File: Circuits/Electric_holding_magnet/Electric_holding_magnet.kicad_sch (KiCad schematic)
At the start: 9 parts, among them J1 Conn_01x03, Q1 BC547, Q2 BC547, SW1 SW_DIP_x01

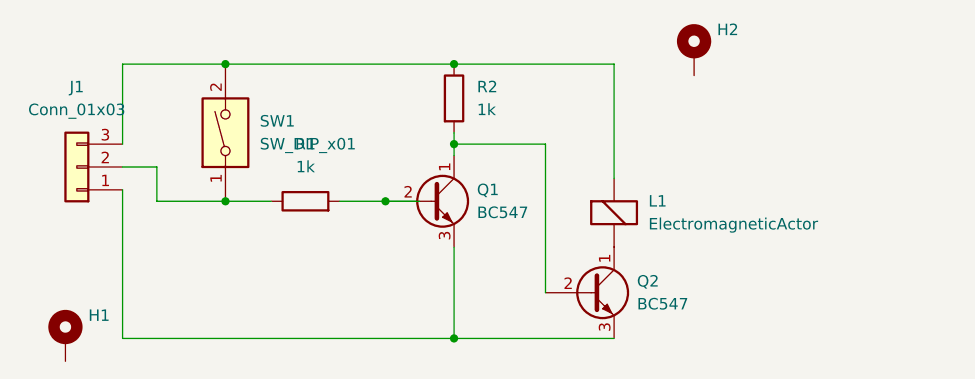
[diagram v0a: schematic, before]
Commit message: udated footprints npn
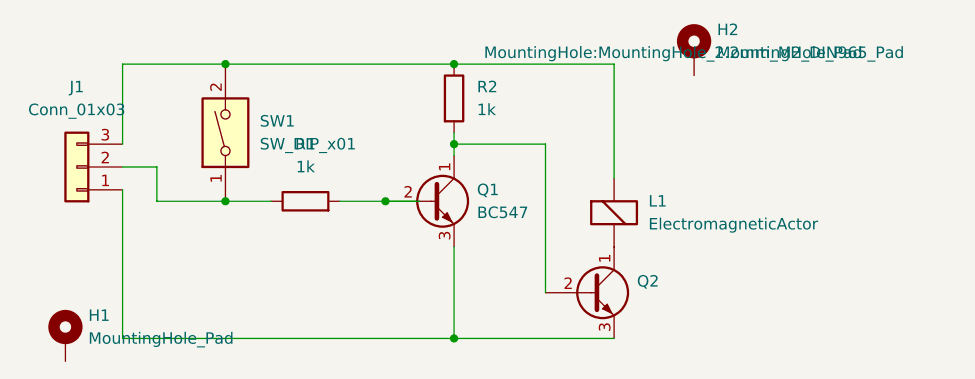
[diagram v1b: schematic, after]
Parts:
- H1, H2: value (none) -> MountingHole_Pad; footprint (none) -> MountingHole:MountingHole_2.2mm_M2_DIN965_Pad
- Q1: footprint Package_TO_SOT_THT:TO-92_Inline -> (none)
- Q2: value BC547 -> (none); footprint Package_TO_SOT_THT:TO-92_Inline -> (none)
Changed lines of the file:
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@@
       (effects (font (size 1.27 1.27)) (justify left))
     )
-    (property "Value" "" (id 1) (at 163.83 64.7699 0)
+    (property "Value" "MountingHole_Pad" (id 1) (at 163.83 64.7699 0)
       (effects (font (size 1.27 1.27)) (justify left))
     )
-    (property "Footprint" "" (id 2) (at 161.29 64.77 0))
+    (property "Footprint" "MountingHole:MountingHole_2.2mm_M2_DIN965_Pad" (id 2) (at 161.29 64.77 0))
     (property "Datasheet" "~" (id 3) (at 161.29 64.77 0)
       (effects (font (size 1.27 1.27)) hide)
@@
       (effects (font (size 1.27 1.27)) (justify left))
     )
-    (property "Footprint" "Package_TO_SOT_THT:TO-92_Inline" (id 2) (at 137.16 83.185 0)
+    (property "Footprint" "" (id 2) (at 137.16 83.185 0)
       (effects (font (size 1.27 1.27) italic) (justify left) hide)
     )
@@
       (effects (font (size 1.27 1.27)) (justify left))
     )
-    (property "Value" "BC547" (id 1) (at 154.94 92.7099 0)
+    (property "Value" "" (id 1) (at 154.94 92.7099 0)
       (effects (font (size 1.27 1.27)) (justify left))
     )
-    (property "Footprint" "Package_TO_SOT_THT:TO-92_Inline" (id 2) (at 154.94 93.345 0)
+    (property "Footprint" "" (id 2) (at 154.94 93.345 0)
       (effects (font (size 1.27 1.27) italic) (justify left) hide)
     )
@@
       (effects (font (size 1.27 1.27)) (justify left))
     )
-    (property "Value" "" (id 1) (at 93.98 96.5199 0)
+    (property "Value" "MountingHole_Pad" (id 1) (at 93.98 96.5199 0)
       (effects (font (size 1.27 1.27)) (justify left))
     )
-    (property "Footprint" "" (id 2) (at 91.44 96.52 0)
+    (property "Footprint" "MountingHole:MountingHole_2.2mm_M2_DIN965_Pad" (id 2) (at 91.44 96.52 0)
       (effects (font (size 1.27 1.27)) hide)
     )
@@
     )
     (path "/7f52d787-caa3-4a92-b1b2-19d554dc29a4"
-      (reference "Q1") (unit 1) (value "BC547") (footprint "Package_TO_SOT_THT:TO-92_Inline")
+      (reference "Q1") (unit 1) (value "BC547") (footprint "Package_TO_SOT_THT:TO-92_HandSolder")
     )
     (path "/90e410ad-8466-4f6d-aba5-640aff7389dc"
-      (reference "Q2") (unit 1) (value "BC547") (footprint "Package_TO_SOT_THT:TO-92_Inline")
+      (reference "Q2") (unit 1) (value "BC547") (footprint "Package_TO_SOT_THT:TO-92_HandSolder")
     )
     (path "/d4fe307e-1033-4241-963d-fdbaaa45a5e9"
